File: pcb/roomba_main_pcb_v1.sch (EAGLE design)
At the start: 14 parts, among them J1 J25MM

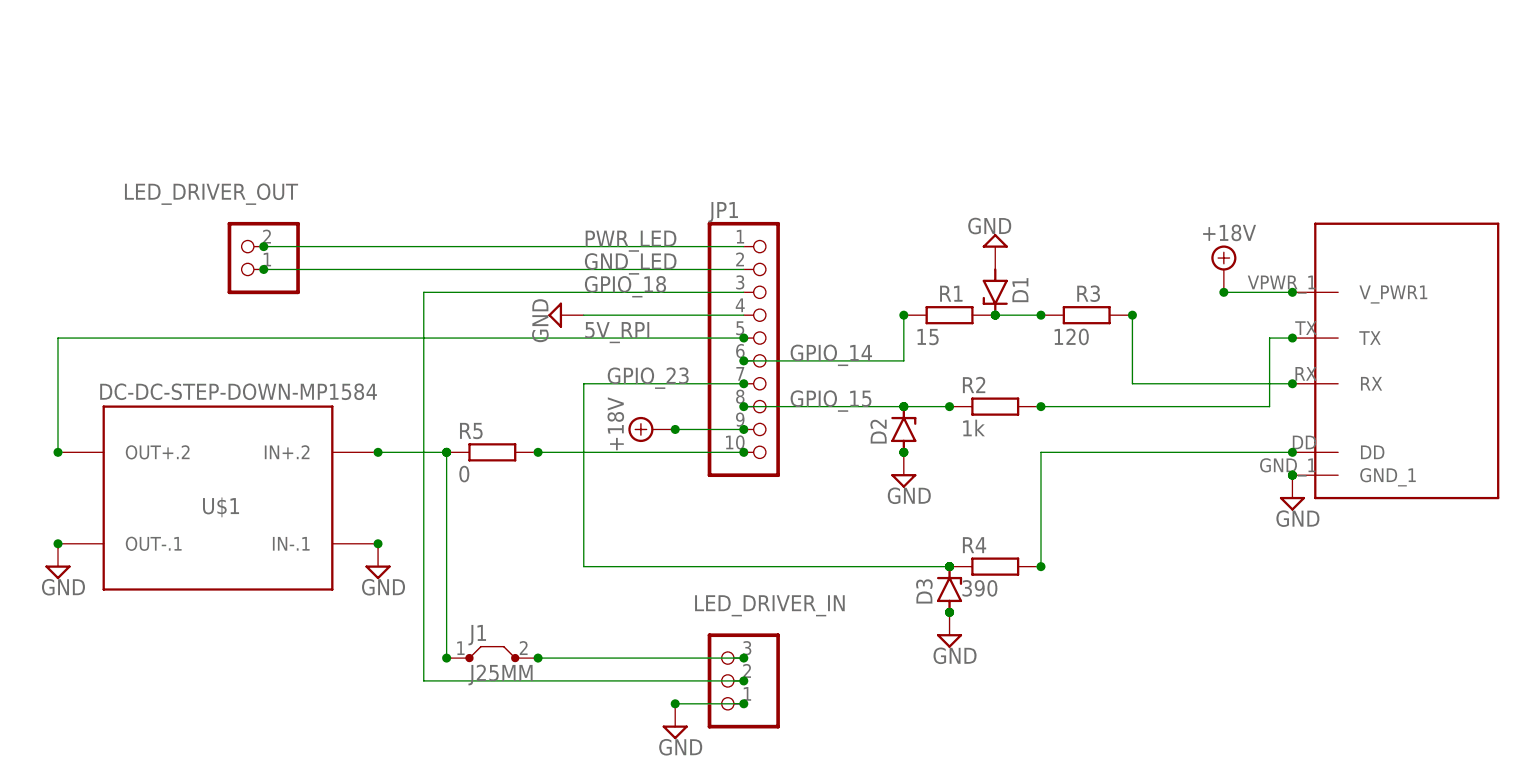
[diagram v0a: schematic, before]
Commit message: 1.1
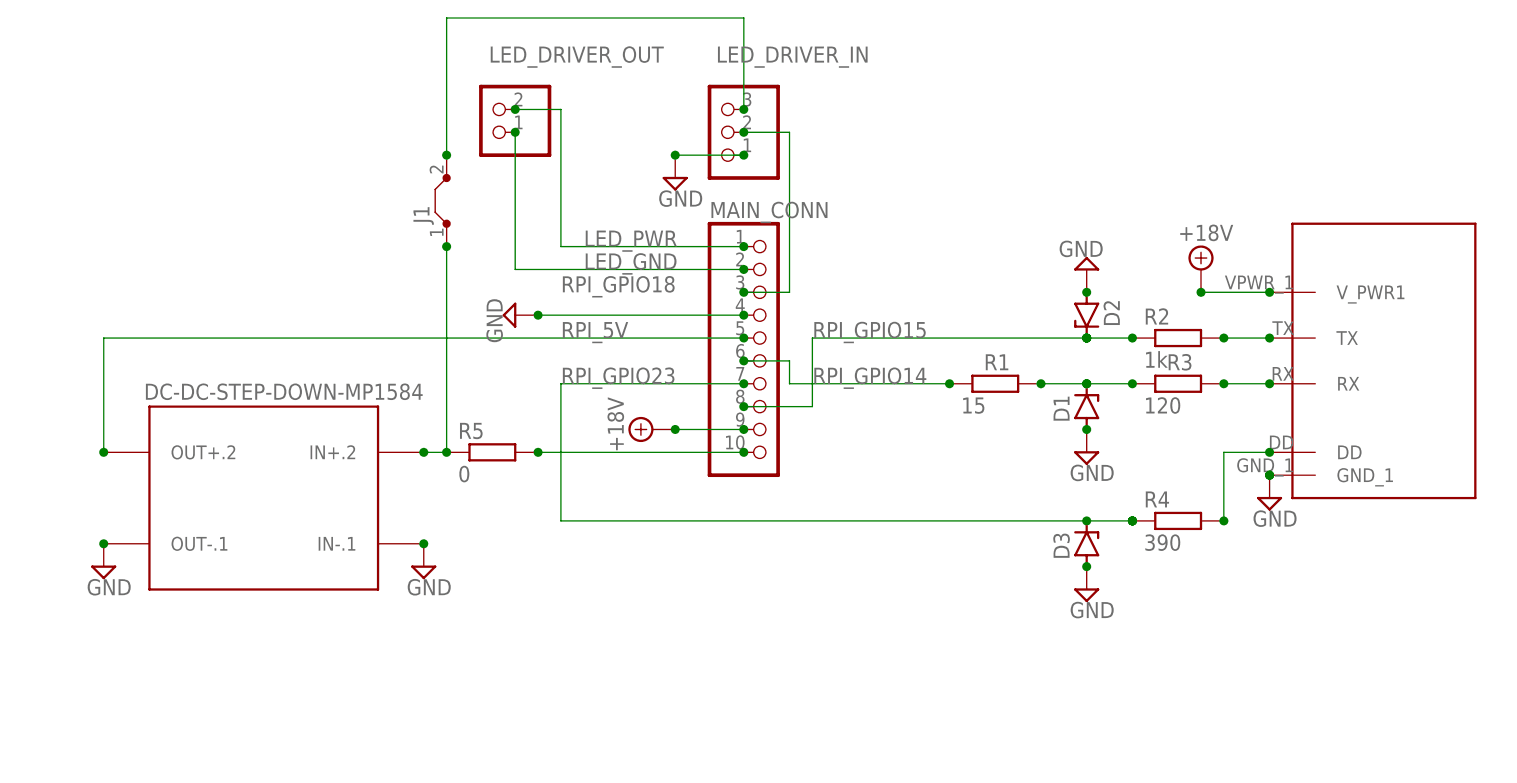
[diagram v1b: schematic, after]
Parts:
- renumbered JP1 to MAIN_CONN
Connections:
- net 5V_RPI renamed RPI_5V
- net GND_LED renamed LED_GND
- net GPIO_14 renamed RPI_GPIO14
- net GPIO_15 renamed RPI_GPIO15
- net GPIO_18 renamed RPI_GPIO18
- net GPIO_23 renamed RPI_GPIO23
- net PWR_LED renamed LED_PWR
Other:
- moved on the sheet: D1, D2, D3, J1, LED_DRIVER_IN, LED_DRIVER_OUT, R1, R2, R3, R4
